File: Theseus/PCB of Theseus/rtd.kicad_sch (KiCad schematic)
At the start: 21 parts, among them J10 Screw_Terminal_01x03, J3 Screw_Terminal_01x03, J9 Screw_Terminal_01x03, U10 INA326, U3 REF200, U4 INA326, U5 INA326, U7 REF200, U9 REF200

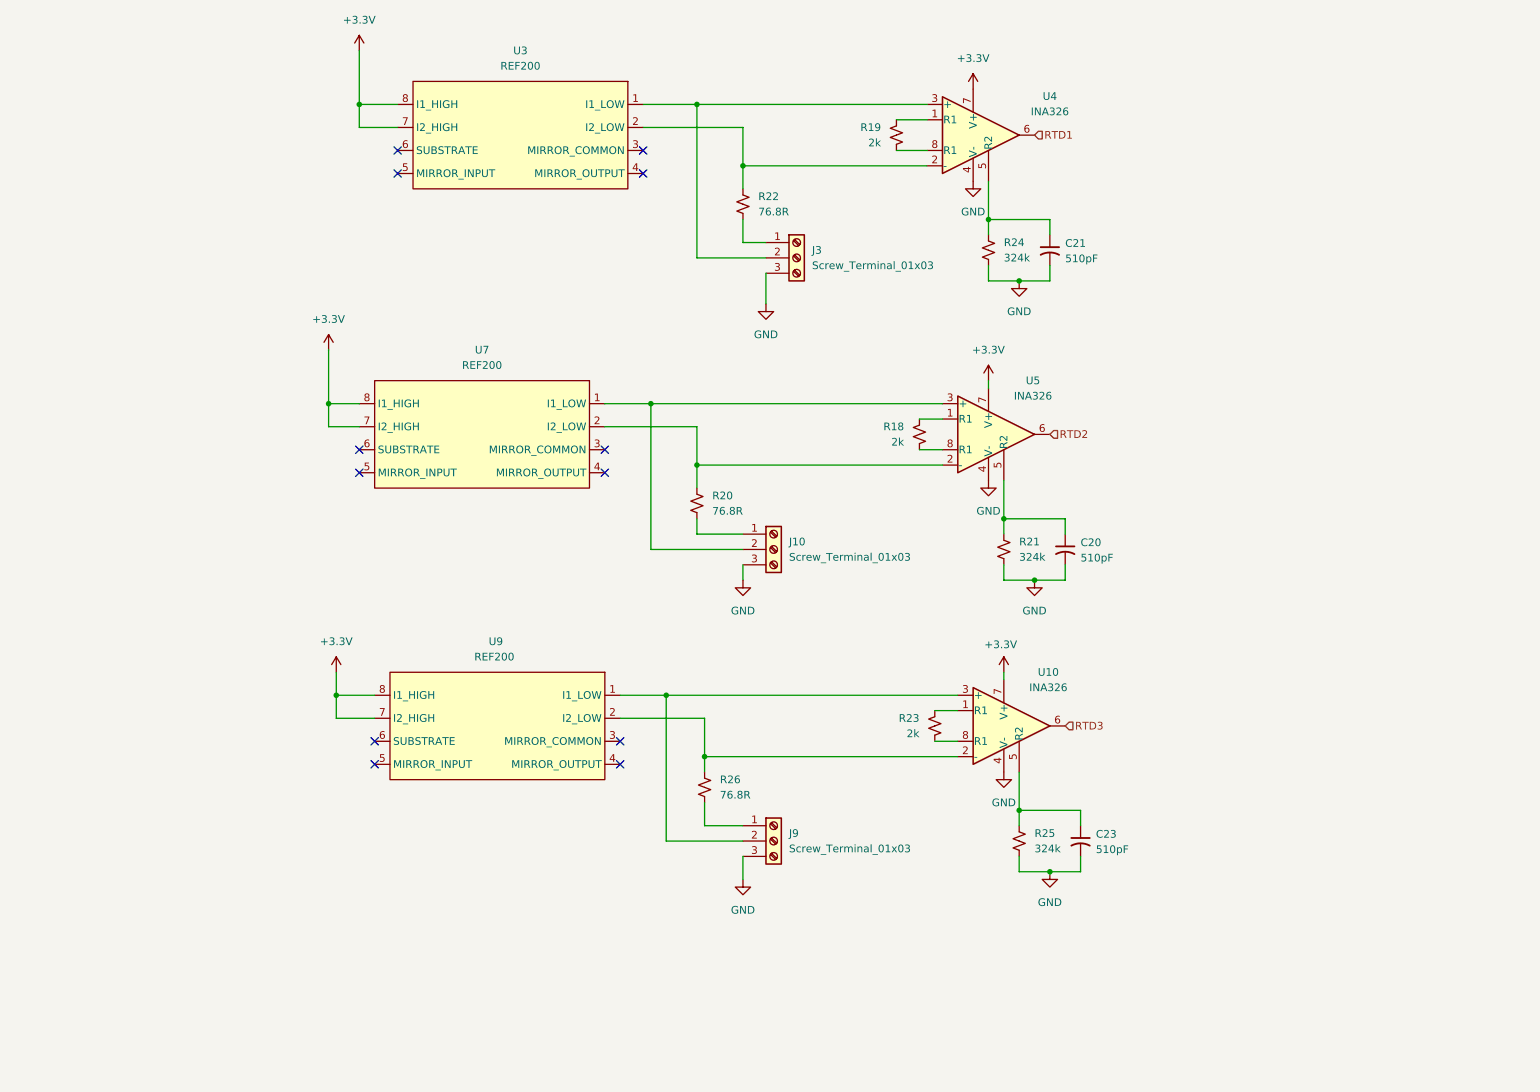
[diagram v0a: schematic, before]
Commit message: Theseus_Dev_Rev2
It's still the same PCB
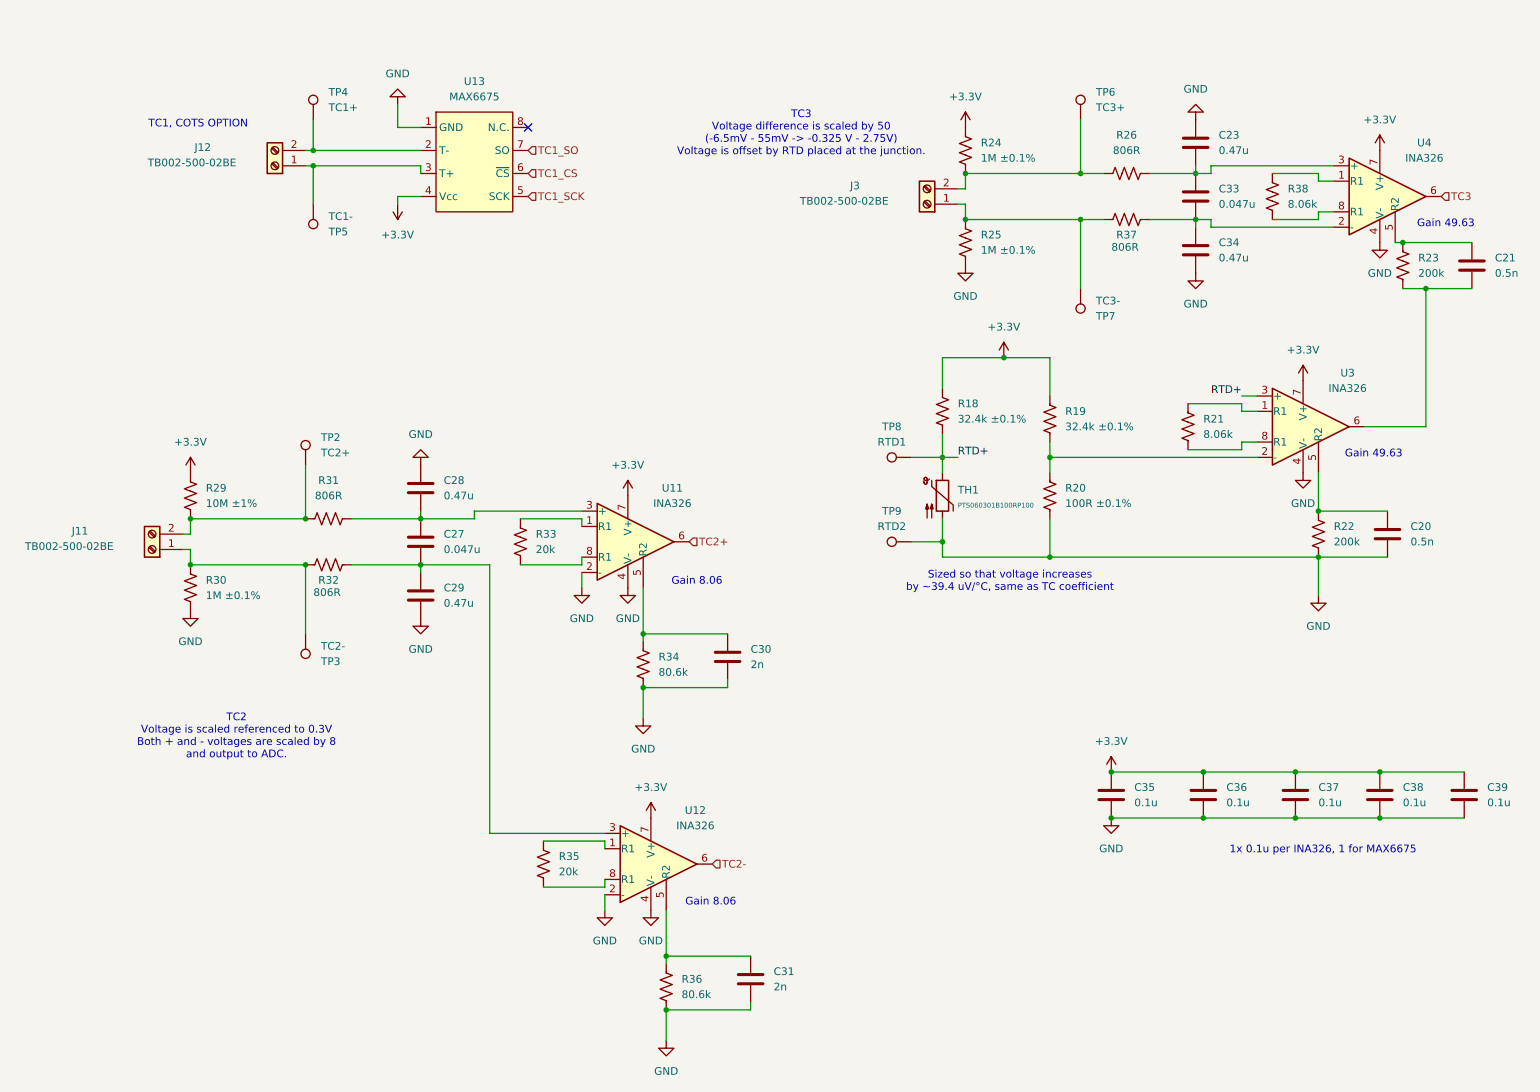
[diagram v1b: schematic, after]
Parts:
- removed C20, C21, C23: 510pF, Capacitor_SMD:C_0201_0603Metric_Pad0.64x0.40mm_HandSolder, symbol Device:C_Small_US
- removed J10, J3, J9: Screw_Terminal_01x03, TerminalBlock_CUI:TerminalBlock_CUI_TB007-508-03_1x03_P5.08mm_Horizontal, symbol Connector:Screw_Terminal_01x03
- removed R18, R19, R23: 2k, Resistor_SMD:R_0603_1608Metric_Pad0.98x0.95mm_HandSolder, symbol Device:R_Small_US
- removed R20, R22, R26: 76.8R, Resistor_SMD:R_0603_1608Metric_Pad0.98x0.95mm_HandSolder, symbol Device:R_Small_US
- removed R21, R24, R25: 324k, Resistor_SMD:R_0201_0603Metric_Pad0.64x0.40mm_HandSolder, symbol Device:R_Small_US
- removed U10, U5: INA326, Package_SO:MSOP-8_3x3mm_P0.65mm, symbol Amplifier_Instrumentation:INA326
- removed U3, U7, U9: REF200, Package_SO:SOIC-8_3.9x4.9mm_P1.27mm, symbol FYDP_Library:REF200
- added C20, C21: 0.5n, Capacitor_SMD:C_0805_2012Metric_Pad1.18x1.45mm_HandSolder, symbol Device:C
- added C23, C28, C29, C34: 0.47u, Capacitor_SMD:C_0805_2012Metric_Pad1.18x1.45mm_HandSolder, symbol Device:C
- added C27, C33: 0.047u, Capacitor_SMD:C_0805_2012Metric_Pad1.18x1.45mm_HandSolder, symbol Device:C
- added C30, C31: 2n, Capacitor_SMD:C_0805_2012Metric_Pad1.18x1.45mm_HandSolder, symbol Device:C
- added C35, C36, C37, C38, C39: 0.1u, Capacitor_SMD:C_0805_2012Metric_Pad1.18x1.45mm_HandSolder, symbol Device:C
- added J11, J12, J3: TB002-500-02BE, TerminalBlock_CUI:TerminalBlock_CUI_TB007-508-02_1x02_P5.08mm_Horizontal, symbol Connector:Screw_Terminal_01x02
- added R18, R19: 32.4k ±0.1%, Resistor_SMD:R_0805_2012Metric_Pad1.20x1.40mm_HandSolder, symbol Device:R_US
- added R20: 100R ±0.1%, Resistor_SMD:R_0805_2012Metric_Pad1.20x1.40mm_HandSolder, symbol Device:R_US
- added R21, R38: 8.06k, Resistor_SMD:R_0805_2012Metric_Pad1.20x1.40mm_HandSolder, symbol Device:R_US
- added R22, R23: 200k, Resistor_SMD:R_0805_2012Metric_Pad1.20x1.40mm_HandSolder, symbol Device:R_US
- added R24, R25, R30: 1M ±0.1%, Resistor_SMD:R_0805_2012Metric_Pad1.20x1.40mm_HandSolder, symbol Device:R_US
- added R26, R31, R32, R37: 806R, Resistor_SMD:R_0805_2012Metric_Pad1.20x1.40mm_HandSolder, symbol Device:R_US
- added R29: 10M ±1%, Resistor_SMD:R_0805_2012Metric_Pad1.20x1.40mm_HandSolder, symbol Device:R_US
- added R33, R35: 20k, Resistor_SMD:R_0805_2012Metric_Pad1.20x1.40mm_HandSolder, symbol Device:R_US
- added R34, R36: 80.6k, Resistor_SMD:R_0805_2012Metric_Pad1.20x1.40mm_HandSolder, symbol Device:R_US
- added TH1: PTS060301B100RP100, Resistor_SMD:R_0603_1608Metric_Pad0.98x0.95mm_HandSolder, symbol Sensor_Temperature:PT100
- added TP2: TC2+, TestPoint:TestPoint_Pad_D2.0mm, symbol Connector:TestPoint
- added TP3: TC2-, TestPoint:TestPoint_Pad_D2.0mm, symbol Connector:TestPoint
- added TP4: TC1+, TestPoint:TestPoint_Pad_D2.0mm, symbol Connector:TestPoint
- added TP5: TC1-, TestPoint:TestPoint_Pad_D2.0mm, symbol Connector:TestPoint
- added TP6: TC3+, TestPoint:TestPoint_Pad_D2.0mm, symbol Connector:TestPoint
- added TP7: TC3-, TestPoint:TestPoint_Pad_D2.0mm, symbol Connector:TestPoint
- added TP8: RTD1, TestPoint:TestPoint_Pad_D2.0mm, symbol Connector:TestPoint
- added TP9: RTD2, TestPoint:TestPoint_Pad_D2.0mm, symbol Connector:TestPoint
- added U11, U12, U3: INA326, Package_SO:MSOP-8_3x3mm_P0.65mm, symbol Amplifier_Instrumentation:INA326
- added U13: MAX6675, Package_SO:SOIC-8_3.9x4.9mm_P1.27mm, symbol FYDP_Library:MAX6675
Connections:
- net +3.3V: now also C35.1, C36.1, C37.1, C38.1, C39.1, R18.1, R19.1, R24.1, R29.1, U11.7 (V+), U12.7 (V+), U13.4 (Vcc), U3.7 (V+)
- net GND: now also C20.2, C23.1, C28.1, C29.2, C30.2, C31.2, C34.2, C35.2, C36.2, C37.2, C38.2, C39.2, R20.2, R22.2, R25.2, R30.2, R34.2, R36.2, TH1.2, TP9.1, U11.2 (-), U11.4 (V-), U12.2 (-), U12.4 (V-), U13.1 (GND), U3.4 (V-)
- net at U4.5 (R2): now also C21.1, R23.1
- net at U4.1 (R1): now also R38.1
- net at U4.2 (-): now also C33.2, C34.1, R37.2
- net at U4.3 (+): now also C23.2, C33.1, R26.2
- net at U4.8 (R1): now also R38.2
- net RTD1 renamed TC3
- new net: J11.2 (Pin_2), R29.2, R31.1, TP2.1
- new net: J12.1 (Pin_1), TP5.1, U13.3 (T+)
- new net: J12.2 (Pin_2), TP4.1, U13.2 (T-)
- new net: C30.1, R34.1, U11.5 (R2)
- new net: C21.2, R23.2, U3.6
- new net: R35.1, U12.1 (R1)
- new net: C27.2, C29.1, R32.2, U12.3 (+)
- new net: C31.1, R36.1, U12.5 (R2)
- new net: R35.2, U12.8 (R1)
- new net: J3.1 (Pin_1), R25.1, R37.1, TP7.1
- new net: J3.2 (Pin_2), R24.2, R26.1, TP6.1
- new net: R19.2, R20.1, U3.2 (-)
- new net: J11.1 (Pin_1), R30.1, R32.1, TP3.1
- new net: C27.1, C28.2, R31.2, U11.3 (+)
- new net: R33.1, U11.1 (R1)
- new net: R33.2, U11.8 (R1)
- new net: C20.1, R22.1, U3.5 (R2)
- new net: R21.1, U3.1 (R1)
- new net: R21.2, U3.8 (R1)
- new net RTD+: R18.2, TH1.1, TP8.1, U3.3 (+)
- new net TC1_CS: U13.6 (~{CS})
- new net TC1_SCK: U13.5 (SCK)
- new net TC1_SO: U13.7 (SO)
- new net TC2+: U11.6
- new net TC2-: U12.6
- no-connect marks 12 -> 1
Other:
- note added: "1x 0.1u per INA326, 1 for MAX6675"
- note added: "Gain 49.63"
- note added: "Gain 8.06"
- note added: "Sized so that voltage increases by ~39.4 uV/°C, same as TC coefficient"
- note added: "TC1, COTS OPTION"
- note added: "TC2 Voltage is scaled referenced to 0.3V Both + and - voltages are scaled by 8 and output to ADC."
- note added: "TC3 Voltage difference is scaled by 50 (-6.5mV - 55mV -> -0.325 V - 2.75V) Voltage is offset by RTD placed at the junction."
